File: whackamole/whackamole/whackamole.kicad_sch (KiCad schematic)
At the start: 18 parts, among them U1 74HC595, U2 CC56-12EWA

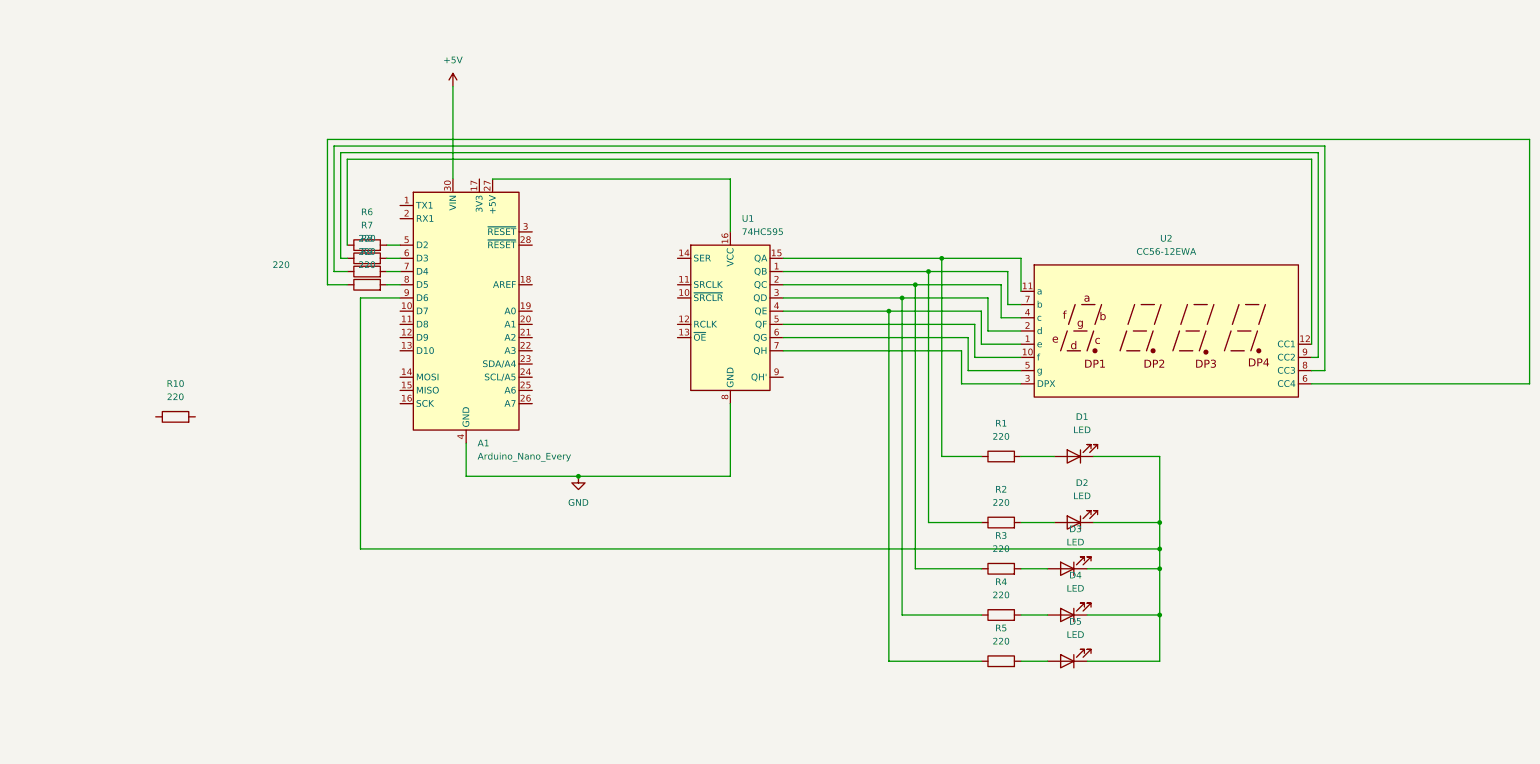
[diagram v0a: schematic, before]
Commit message: progress, yeah
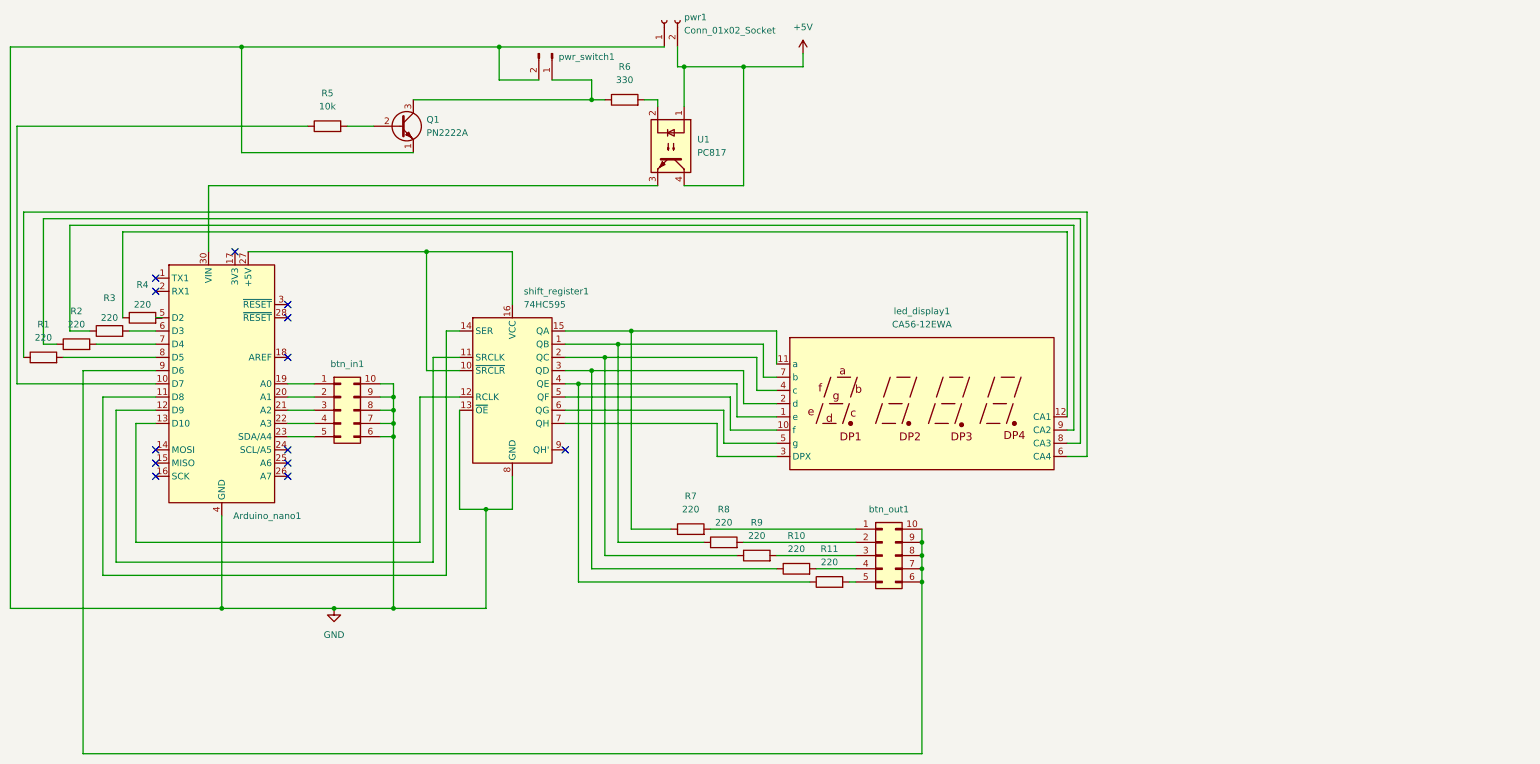
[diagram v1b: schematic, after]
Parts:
- removed D1, D2, D3, D4, D5: LED, LED_THT:LED_D1.8mm_W3.3mm_H2.4mm, symbol Device:LED
- removed R10: 220, Resistor_THT:R_Axial_DIN0204_L3.6mm_D1.6mm_P1.90mm_Vertical, symbol Device:R
- removed U2: CC56-12EWA, Package_DIP:DIP-16_W7.62mm, symbol Display_Character:CC56-12EWA
- added Q1: PN2222A, Package_TO_SOT_THT:TO-92, symbol Transistor_BJT:PN2222A
- added R5: 10k, Resistor_THT:R_Axial_DIN0207_L6.3mm_D2.5mm_P2.54mm_Vertical, symbol Device:R
- added R6: 330, Resistor_THT:R_Axial_DIN0204_L3.6mm_D1.6mm_P1.90mm_Vertical, symbol Device:R
- added U1: PC817, Package_DIP:DIP-4_W7.62mm, symbol Isolator:PC817
- added btn_in1, btn_out1: ~, Connector_PinHeader_2.54mm:PinHeader_2x05_P2.54mm_Vertical, symbol Connector_Generic:Conn_02x05_Counter_Clockwise
- added led_display1: CA56-12EWA, Display_7Segment:CA56-12EWA, symbol Display_Character:CA56-12EWA
- added pwr1: Conn_01x02_Socket, Connector_PinSocket_1.27mm:PinSocket_1x02_P1.27mm_Vertical, symbol Connector:Conn_01x02_Socket
- added pwr_switch1: ~, Connector_PinHeader_2.54mm:PinHeader_1x02_P2.54mm_Vertical, symbol Connector:Conn_01x02_Pin
- Arduino_nano1: renamed from A1; value Arduino_Nano_Every -> ~
- renumbered R9 to R1, R4 to R10, R5 to R11, R8 to R2, R7 to R3, R6 to R4, R1 to R7, R2 to R8, R3 to R9, U1 to shift_register1
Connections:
- net +5V: now also U1.1, U1.4, pwr1.2 (Pin_2); no longer Arduino_nano1.30 (VIN)
- net GND: now also shift_register1.13 (~{OE}), Q1.1 (E), btn_in1.10 (Pin_10), btn_in1.6 (Pin_6), btn_in1.7 (Pin_7), btn_in1.8 (Pin_8), btn_in1.9 (Pin_9), pwr1.1 (Pin_1), pwr_switch1.2 (Pin_2)
- net at Arduino_nano1.9 (D6): now also btn_out1.10 (Pin_10), btn_out1.6 (Pin_6), btn_out1.7 (Pin_7), btn_out1.8 (Pin_8), btn_out1.9 (Pin_9)
- net at R10.2: now also btn_out1.4 (Pin_4)
- net at Arduino_nano1.10 (D7): now also R5.1
- net at Arduino_nano1.11 (D8): now also shift_register1.14 (SER)
- net at Arduino_nano1.12 (D9): now also shift_register1.11 (SRCLK)
- net at Arduino_nano1.13 (D10): now also shift_register1.12 (RCLK)
- net at Arduino_nano1.19 (A0): now also btn_in1.1 (Pin_1)
- net at Arduino_nano1.20 (A1): now also btn_in1.2 (Pin_2)
- net at Arduino_nano1.21 (A2): now also btn_in1.3 (Pin_3)
- net at Arduino_nano1.22 (A3): now also btn_in1.4 (Pin_4)
- net at Arduino_nano1.23 (SDA/A4): now also btn_in1.5 (Pin_5)
- net at Arduino_nano1.27 (+5V), shift_register1.16 (VCC): now also shift_register1.10 (~{SRCLR})
- net at R9.2: now also btn_out1.3 (Pin_3)
- net at R8.2: now also btn_out1.2 (Pin_2)
- net at R7.1, shift_register1.15 (QA): now also led_display1.11 (a)
- net at R7.2: now also btn_out1.1 (Pin_1)
- net at R10.1, shift_register1.3 (QD): now also led_display1.2 (d)
- net at R11.1, shift_register1.4 (QE): now also led_display1.1 (e)
- net at shift_register1.5 (QF): now also led_display1.10 (f)
- net at R4.1: now also led_display1.12 (CA1)
- net at shift_register1.7 (QH): now also led_display1.3 (DPX)
- net at R9.1, shift_register1.2 (QC): now also led_display1.4 (c)
- net at shift_register1.6 (QG): now also led_display1.5 (g)
- net at R1.1: now also led_display1.6 (CA4)
- net at R8.1, shift_register1.1 (QB): now also led_display1.7 (b)
- net at R2.1: now also led_display1.8 (CA3)
- net at R3.1: now also led_display1.9 (CA2)
- net at R11.2: now also btn_out1.5 (Pin_5)
- new net: Arduino_nano1.30 (VIN), U1.3
- new net: Q1.2 (B), R5.2
- new net: R6.2, U1.2
- new net: Q1.3 (C), R6.1, pwr_switch1.1 (Pin_1)
- no-connect marks 0 -> 13
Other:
- moved on the sheet: Arduino_nano1, R1, R10, R11, R2, R3, R4, R7, R8, R9, shift_register1
